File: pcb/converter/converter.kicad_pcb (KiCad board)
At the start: 2 copper layers, 26.5 x 16 mm, 8 parts, among them J1 BMS_DATA, J2 BMS_GND, J3 ESP_GND, J4 ESP_DATA, J5 ESP_VCC, U1 PC817

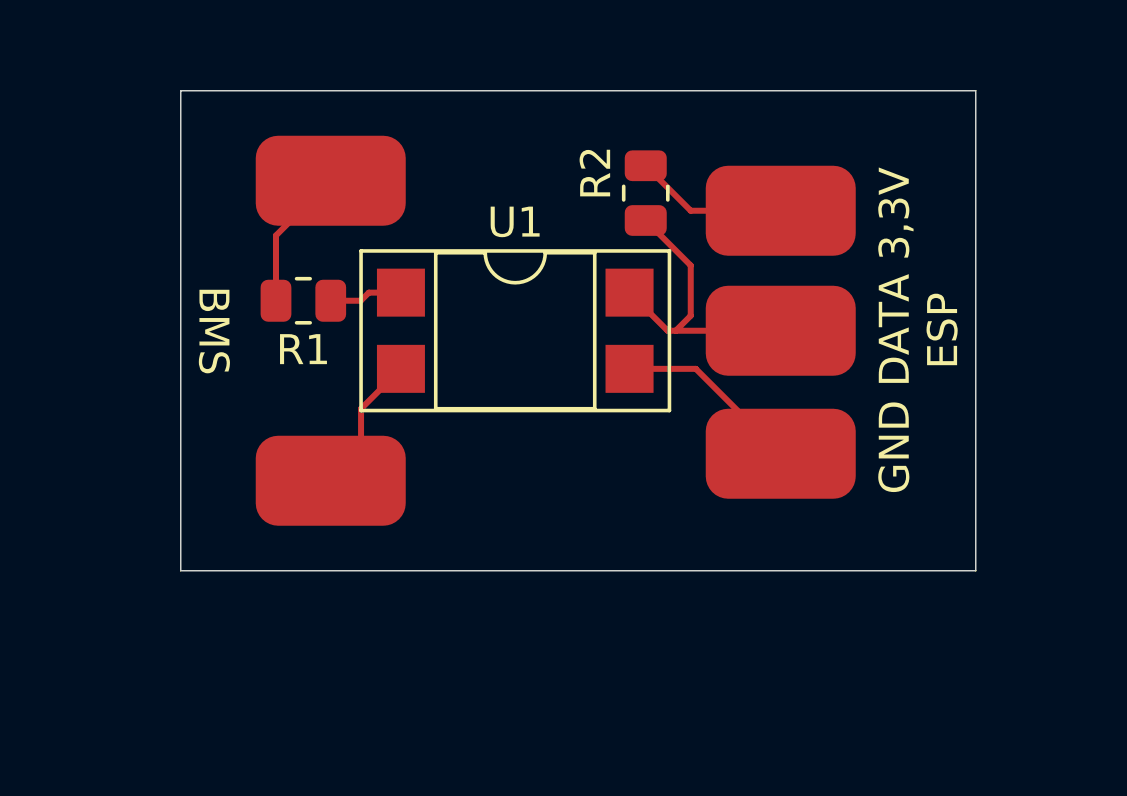
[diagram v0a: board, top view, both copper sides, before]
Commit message: edited pcb
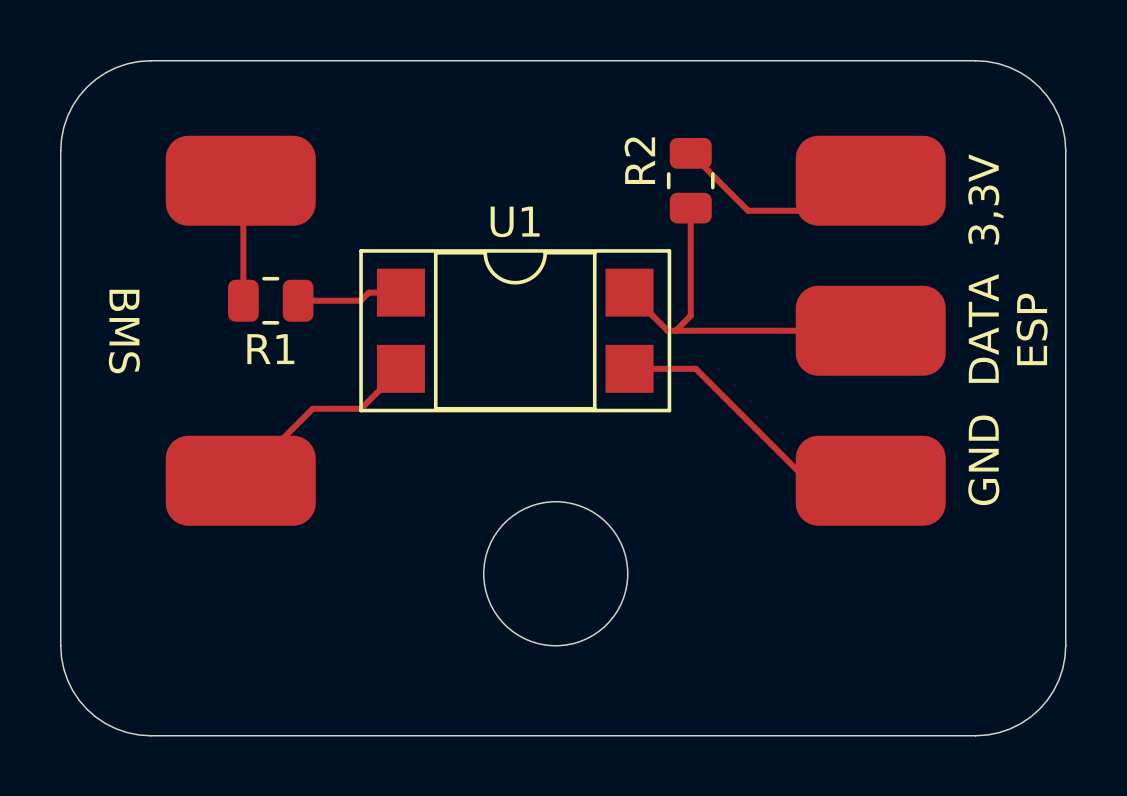
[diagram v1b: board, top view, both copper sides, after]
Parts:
- moved J5 3.16 mm to (69.0, 20.0)
- moved J3 3.13 mm to (69.0, 30.0)
- moved J1 3.00 mm to (48.0, 20.0)
- moved J2 3.00 mm to (48.0, 30.0)
- moved J4 3.00 mm to (69.0, 25.0)
- moved R2 1.56 mm to (63.0, 25.0)
- moved R1 1.09 mm to (49.0, 29.0)
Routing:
- net Net-(J3-Pin_1): track 6.21 -> 9.59 mm
- net Net-(J4-Pin_1): track 10.1 -> 12.9 mm
- net Net-(J2-Pin_1): track 4.70 -> 6.89 mm
- net Net-(J5-Pin_1): track 5.12 -> 7.21 mm
- net Net-(R1-Pad1): track 2.45 -> 3.54 mm
- net Net-(J1-Pin_1): track 4.76 -> 4.04 mm
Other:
- board size 26.5 x 16 mm -> 33.5 x 22.5 mm
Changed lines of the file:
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@@
 	(footprint "Custom:SolderPad5x3mm"
 		(layer "F.Cu")
-		(at 66 25)
+		(at 69 25)
 		(property "Reference" "J4"
 			(at 0 -0.5 0)
@@
 	(footprint "Custom:SolderPad5x3mm"
 		(layer "F.Cu")
-		(at 51 20)
+		(at 48 20)
 		(property "Reference" "J1"
 			(at 3.5 3.4 0)
@@
 	(footprint "Custom:SolderPad5x3mm"
 		(layer "F.Cu")
-		(at 66 29.1)
+		(at 69 30)
 		(property "Reference" "J3"
 			(at 0 -0.5 0)
@@
 				(font
 					(size 1.27 1.27)
+					(thickness 0.15)
 				)
 			)
@@
 				(font
 					(size 1.27 1.27)
+					(thickness 0.15)
 				)
 			)
@@
 				(font
 					(size 1.27 1.27)
+					(thickness 0.15)
 				)
 			)
@@
 	(footprint "Custom:SolderPad5x3mm"
 		(layer "F.Cu")
-		(at 51 30)
+		(at 48 30)
 		(property "Reference" "J2"
 			(at 3.5 6.4 0)
@@
 	(footprint "Custom:SolderPad5x3mm"
 		(layer "F.Cu")
-		(at 66 21)
+		(at 69 20)
 		(property "Reference" "J5"
 			(at 0 7.5 0)
@@
 	(footprint "Resistor_SMD:R_0805_2012Metric"
 		(layer "F.Cu")
-		(at 61.5 25.4125 90)
+		(at 63 25 90)
 		(descr "Resistor SMD 0805 (2012 Metric), square (rectangular) end terminal, IPC_7351 nominal, (Body size source: IPC-SM-782 page 72, https://www.pcb-3d.com/wordpress/wp-content/uploads/ipc-sm-782a_amendment_1_and_2.pdf), generated with kicad-footprint-generator")
 		(tags "resistor")
@@
 				(font
 					(size 1.27 1.27)
+					(thickness 0.15)
 				)
 			)
@@
 				(font
 					(size 1.27 1.27)
+					(thickness 0.15)
 				)
 			)
@@
 				(font
 					(size 1.27 1.27)
+					(thickness 0.15)
 				)
 			)
@@
 	(footprint "Resistor_SMD:R_0805_2012Metric"
 		(layer "F.Cu")
-		(at 50.0875 29 180)
+		(at 49 29 180)
 		(descr "Resistor SMD 0805 (2012 Metric), square (rectangular) end terminal, IPC_7351 nominal, (Body size source: IPC-SM-782 page 72, https://www.pcb-3d.com/wordpress/wp-content/uploads/ipc-sm-782a_amendment_1_and_2.pdf), generated with kicad-footprint-generator")
 		(tags "resistor")
@@
 				(font
 					(size 1.27 1.27)
+					(thickness 0.15)
 				)
 			)
@@
 				(font
 					(size 1.27 1.27)
+					(thickness 0.15)
 				)
 			)
@@
 				(font
 					(size 1.27 1.27)
+					(thickness 0.15)
 				)
 			)
@@
 		)
 	)
-	(gr_rect
-		(start 46 22)
-		(end 72.5 38)
+	(gr_arc
+		(start 72.5 21)
+		(mid 74.62132 21.87868)
+		(end 75.5 24)
 		(stroke
 			(width 0.05)
 			(type default)
 		)
+		(layer "Edge.Cuts")
+	)
+	(gr_line
+		(start 75.5 24)
+		(end 75.5 40.5)
+		(stroke
+			(width 0.05)
+			(type default)
+		)
+		(layer "Edge.Cuts")
+	)
+	(gr_line
+		(start 42 40.5)
+		(end 42 24)
+		(stroke
+			(width 0.05)
+			(type default)
+		)
+		(layer "Edge.Cuts")
+	)
+	(gr_arc
+		(start 45 43.5)
+		(mid 42.87868 42.62132)
+		(end 42 40.5)
+		(stroke
+			(width 0.05)
+			(type default)
+		)
+		(layer "Edge.Cuts")
+	)
+	(gr_line
+		(start 72.5 43.5)
+		(end 45 43.5)
+		(stroke
+			(width 0.05)
+			(type default)
+		)
+		(layer "Edge.Cuts")
+	)
+	(gr_line
+		(start 72.5 21)
+		(end 45 21)
+		(stroke
+			(width 0.05)
+			(type default)
+		)
+		(layer "Edge.Cuts")
+	)
+	(gr_arc
+		(start 75.5 40.5)
+		(mid 74.62132 42.62132)
+		(end 72.5 43.5)
+		(stroke
+			(width 0.05)
+			(type default)
+		)
+		(layer "Edge.Cuts")
+	)
+	(gr_arc
+		(start 42 24)
+		(mid 42.87868 21.87868)
+		(end 45 21)
+		(stroke
+			(width 0.05)
+			(type default)
+		)
+		(layer "Edge.Cuts")
+	)
+	(gr_circle
+		(center 58.5 38.1)
+		(end 60.9 38.1)
+		(stroke
+			(width 0.05)
+			(type default)
+		)
 		(fill none)
 		(layer "Edge.Cuts")
 	)
 	(gr_text "BMS"
-		(at 46.5 28.5 270)
+		(at 43.5 28.5 270)
 		(layer "F.SilkS")
 		(effects
@@
 		)
 	)
-	(gr_text "GND DATA 3,3V\nESP"
-		(at 72 30 90)
+	(gr_text "GND  DATA  3,3V\nESP"
+		(at 75 30 90)
 		(layer "F.SilkS")
 		(effects
@@
 	)
 	(segment
-		(start 51 25)
-		(end 49.175 26.825)
+		(start 48 25)
+		(end 48.0875 25.0875)
 		(width 0.2)
 		(layer "F.Cu")
@@
 	)
 	(segment
-		(start 49.175 26.825)
-		(end 49.175 29)
+		(start 48.0875 25.0875)
+		(end 48.0875 29)
 		(width 0.2)
 		(layer "F.Cu")
 		(net 1)
-	)
-	(segment
-		(start 51 35)
-		(end 52.01 33.99)
-		(width 0.2)
-		(layer "F.Cu")
-		(net 2)
 	)
 	(segment
@@
 	)
 	(segment
-		(start 52.01 33.99)
+		(start 50.4 32.6)
 		(end 52.01 32.6)
+		(width 0.2)
+		(layer "F.Cu")
+		(net 2)
+	)
+	(segment
+		(start 48 35)
+		(end 50.4 32.6)
 		(width 0.2)
 		(layer "F.Cu")
@@
 	)
 	(segment
-		(start 51 29)
+		(start 49.9125 29)
 		(end 52 29)
 		(width 0.2)
@@
 	)
 	(segment
-		(start 63 27.825)
+		(start 62.5 30)
+		(end 62.23 30)
+		(width 0.2)
+		(layer "F.Cu")
+		(net 4)
+	)
+	(segment
+		(start 62.23 30)
+		(end 60.96 28.73)
+		(width 0.2)
+		(layer "F.Cu")
+		(net 4)
+	)
+	(segment
+		(start 63 25.9125)
 		(end 63 29.5)
 		(width 0.2)
@@
 	)
 	(segment
-		(start 62.5 30)
-		(end 62.23 30)
+		(start 69 30)
+		(end 62.5 30)
 		(width 0.2)
 		(layer "F.Cu")
@@
 	)
 	(segment
-		(start 62.23 30)
-		(end 60.96 28.73)
-		(width 0.2)
-		(layer "F.Cu")
-		(net 4)
-	)
-	(segment
-		(start 61.5 26.325)
-		(end 63 27.825)
-		(width 0.2)
-		(layer "F.Cu")
-		(net 4)
-	)
-	(segment
-		(start 66 30)
-		(end 62.5 30)
-		(width 0.2)
-		(layer "F.Cu")
-		(net 4)
-	)
-	(segment
-		(start 66 26)
-		(end 63 26)
+		(start 69 25)
+		(end 68 26)
 		(width 0.2)
 		(layer "F.Cu")
@@
 	)
 	(segment
-		(start 63 26)
-		(end 61.5 24.5)
+		(start 68 26)
+		(end 64.9125 26)
 		(width 0.2)
 		(layer "F.Cu")
@@
 	)
 	(segment
-		(start 66 34.1)
-		(end 63.17 31.27)
-		(width 0.2)
-		(layer "F.Cu")
-		(net 6)
+		(start 64.9125 26)
+		(end 63 24.0875)
+		(width 0.2)
+		(layer "F.Cu")
+		(net 5)
 	)
 	(segment
@@
 		(width 0.2)
 		(layer "F.Cu")
+		(net 6)
+	)
+	(segment
+		(start 66.9 35)
+		(end 63.17 31.27)
+		(width 0.2)
+		(layer "F.Cu")
+		(net 6)
+	)
+	(segment
+		(start 69 35)
+		(end 66.9 35)
+		(width 0.2)
+		(layer "F.Cu")
